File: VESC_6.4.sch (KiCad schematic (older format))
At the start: 23 parts, among them J1 CAN, J2 HALL_ENC, J3 COMM, J4 SERVO, J5 SWD, J6 USB_OTG, SW1 SENSOR_VOLTAGE

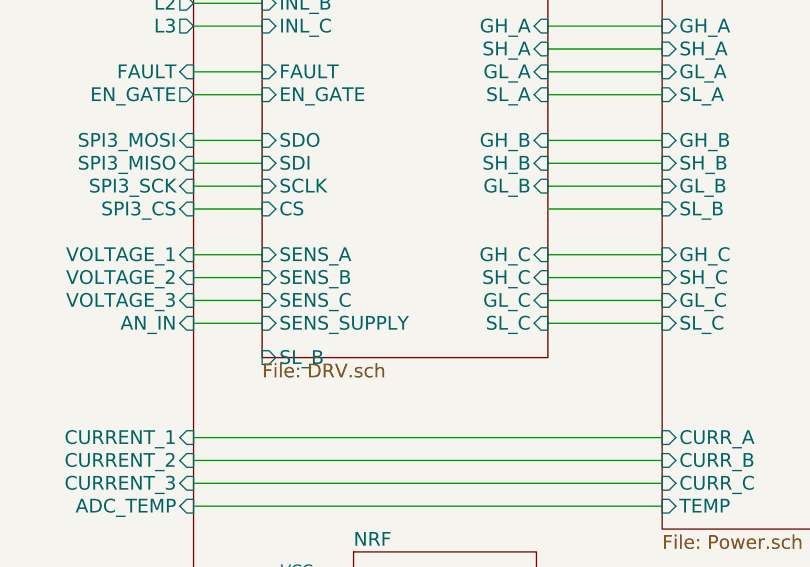
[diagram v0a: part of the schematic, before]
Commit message: lots of PCB work
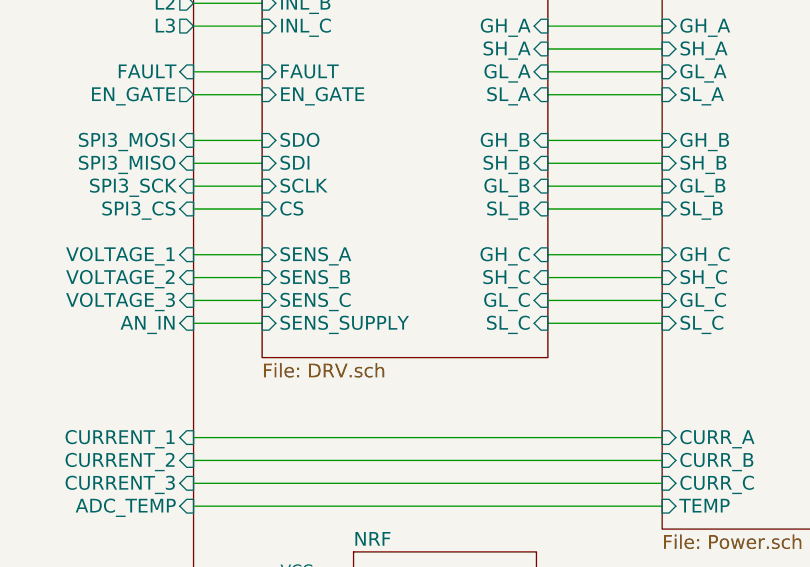
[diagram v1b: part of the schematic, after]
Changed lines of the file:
@@
 F25 "GH_B" I R 8400 2800 60
 F26 "GL_B" I R 8400 3000 60
-F27 "SL_B" I L 7150 3750 60
+F27 "SL_B" I R 8400 3100 60
 F28 "GH_C" I R 8400 3300 60
 F29 "GL_C" I R 8400 3500 60
